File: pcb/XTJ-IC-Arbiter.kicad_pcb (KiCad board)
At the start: 2 copper layers, 80.2 x 67.8 mm, 56 parts, among them IC1 SN74LV125AN, J3 DTM13-12PA-R008, Q1 NPN, U1 LM2675N-5.0/NOPB, U2 CDP68HC68S1, U3 EEC-325X4A, U4 MCP2562-H-P, U5 SP723APP, U6 MCP1700-3302E/TO

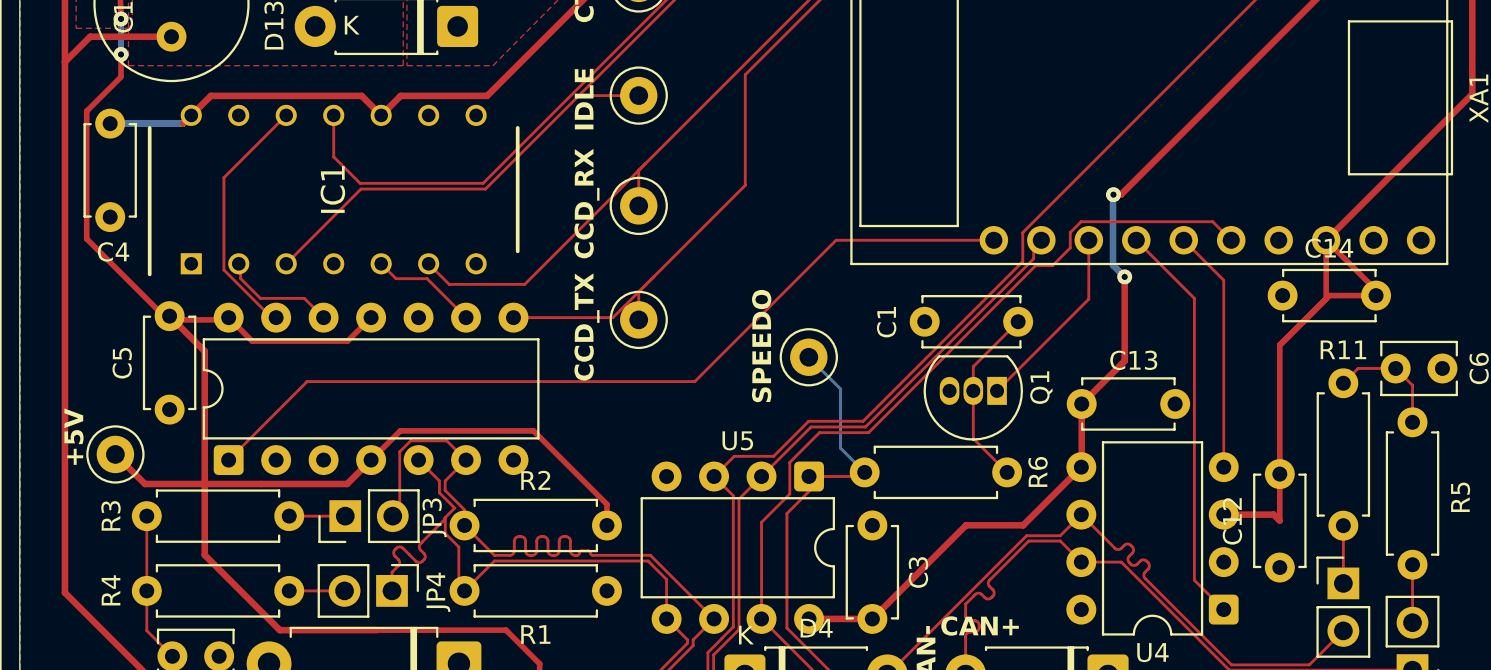
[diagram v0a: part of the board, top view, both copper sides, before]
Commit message: colorize crucial nets
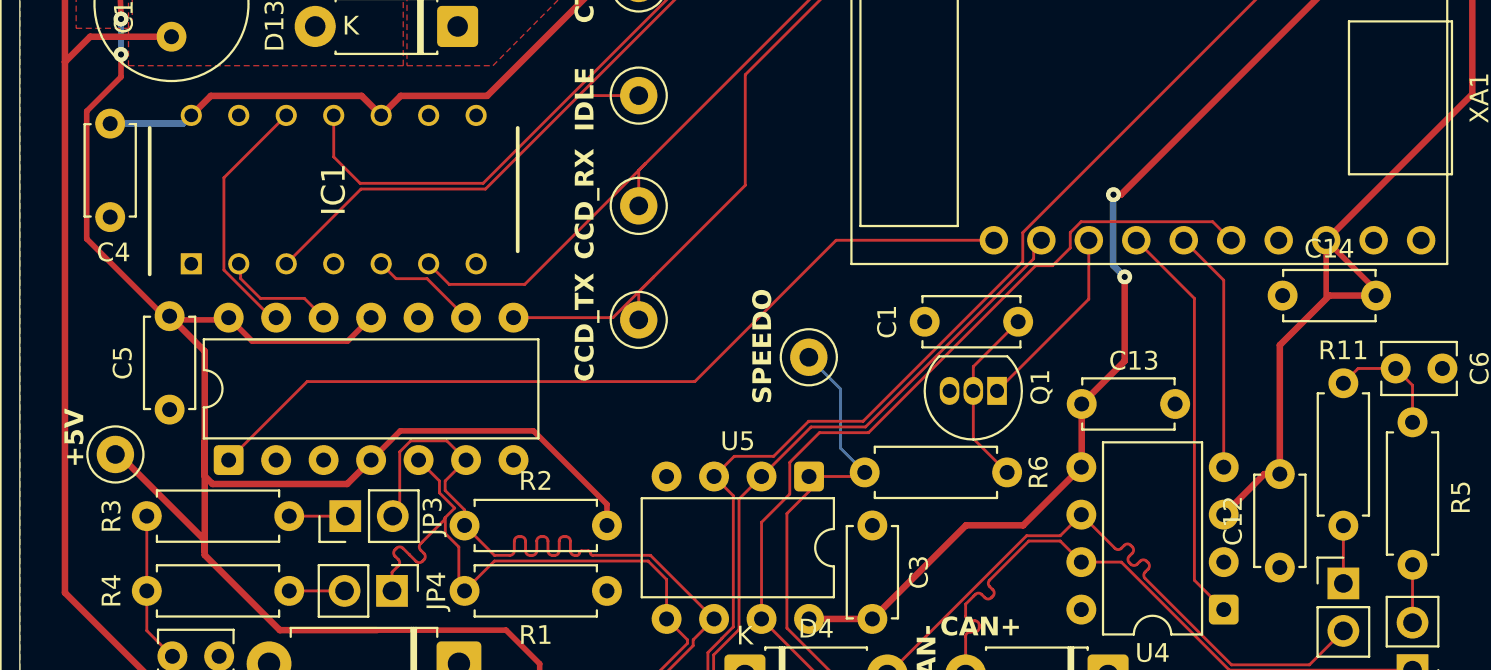
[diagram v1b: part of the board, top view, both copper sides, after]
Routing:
- net +5V: track 239.0 -> 240.9 mm
- net +3V3: track 140.2 -> 139.6 mm
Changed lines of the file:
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@@
-	)
-	(segment
-		(start 170.65 93.7)
-		(end 168 96.35)
-		(width 0.3)
-		(layer "F.Cu")
-		(net 11)
 	)
 	(segment
@@
 	)
 	(segment
+		(start 110.4792 107.4)
+		(end 110.4792 106.787875)
+		(width 0.35)
+		(layer "F.Cu")
+		(net 11)
+	)
+	(segment
 		(start 178.3 82.92)
 		(end 170.48 90.74)
@@
 	)
 	(segment
-		(start 113.5 103.7808)
-		(end 118.0992 103.7808)
+		(start 110.4792 101.5)
+		(end 110.4792 107.4)
 		(width 0.35)
 		(layer "F.Cu")
@@
 	)
 	(segment
-		(start 167.67 105.42)
-		(end 168 105.75)
+		(start 110.4792 107.4)
+		(end 110.4792 107.582189)
 		(width 0.35)
 		(layer "F.Cu")
@@
 	)
 	(segment
-		(start 168 96.35)
-		(end 168 105.75)
-		(width 0.3)
-		(layer "F.Cu")
-		(net 11)
-	)
-	(segment
 		(start 176.7 61.8)
 		(end 178.3 63.4)
@@
 	)
 	(segment
+		(start 165 105.42)
+		(end 167.17 103.25)
+		(width 0.35)
+		(layer "F.Cu")
+		(net 11)
+	)
+	(segment
 		(start 167.515 61.8)
 		(end 176.7 61.8)
@@
 	)
 	(segment
-		(start 173.15 93.7)
-		(end 170.65 93.7)
-		(width 0.3)
+		(start 110.4792 103.359634)
+		(end 110.900366 103.7808)
+		(width 0.35)
+		(layer "F.Cu")
+		(net 11)
+	)
+	(segment
+		(start 118.0992 103.7808)
+		(end 119.38 102.5)
+		(width 0.35)
 		(layer "F.Cu")
 		(net 11)
@@
 	)
 	(segment
-		(start 173.15 93.41)
+		(start 170.65 93.7)
 		(end 173.15 93.7)
-		(width 0.3)
+		(width 0.35)
 		(layer "F.Cu")
 		(net 11)
@@
 	)
 	(segment
-		(start 105.7 102.2)
-		(end 107.2808 103.7808)
-		(width 0.35)
-		(layer "F.Cu")
-		(net 11)
-	)
-	(segment
 		(start 136.03 121.8)
 		(end 138.73 124.5)
@@
 	)
 	(segment
-		(start 107.2808 103.7808)
-		(end 113.5 103.7808)
-		(width 0.35)
-		(layer "F.Cu")
-		(net 11)
-	)
-	(segment
 		(start 104.1642 83.8358)
 		(end 104.1642 90.6642)
@@
 	)
 	(segment
+		(start 168 96.35)
+		(end 170.65 93.7)
+		(width 0.35)
+		(layer "F.Cu")
+		(net 11)
+	)
+	(segment
 		(start 118.1242 96.1358)
 		(end 119.38 94.88)
@@
 	)
 	(segment
+		(start 167.17 103.25)
+		(end 168 103.25)
+		(width 0.35)
+		(layer "F.Cu")
+		(net 11)
+	)
+	(segment
+		(start 168 103.25)
+		(end 168 96.35)
+		(width 0.35)
+		(layer "F.Cu")
+		(net 11)
+	)
+	(segment
 		(start 161.115 68.2)
 		(end 133.8 68.2)
@@
 	(segment
 		(start 110.4792 96.6792)
-		(end 110.4792 107.582189)
+		(end 110.4792 101.5)
 		(width 0.35)
 		(layer "F.Cu")
@@
 	)
 	(segment
-		(start 118.0992 103.7808)
-		(end 119.38 102.5)
+		(start 110.4792 101.5)
+		(end 110.4792 103.359634)
 		(width 0.35)
 		(layer "F.Cu")
@@
 	)
 	(segment
-		(start 165 105.42)
-		(end 167.67 105.42)
-		(width 0.35)
-		(layer "F.Cu")
-		(net 11)
-	)
-	(segment
 		(start 126.6 111.6)
 		(end 128.4 113.4)
@@
 	)
 	(segment
+		(start 105.891325 102.2)
+		(end 105.7 102.2)
+		(width 0.35)
+		(layer "F.Cu")
+		(net 11)
+	)
+	(segment
+		(start 110.900366 103.7808)
+		(end 118.0992 103.7808)
+		(width 0.35)
+		(layer "F.Cu")
+		(net 11)
+	)
+	(segment
 		(start 120.9416 100.9384)
 		(end 119.38 102.5)
 		(width 0.3)
+		(layer "F.Cu")
+		(net 11)
+	)
+	(segment
+		(start 110.4792 106.787875)
+		(end 105.891325 102.2)
+		(width 0.35)
 		(layer "F.Cu")
 		(net 11)
@@
 		(width 0.35)
 		(layer "F.Cu")
-		(net 13)
-	)
-	(segment
-		(start 109.76 84.06)
-		(end 109.32 84.5)
-		(width 0.35)
-		(layer "F.Cu")
